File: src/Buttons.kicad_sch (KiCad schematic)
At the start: 23 parts

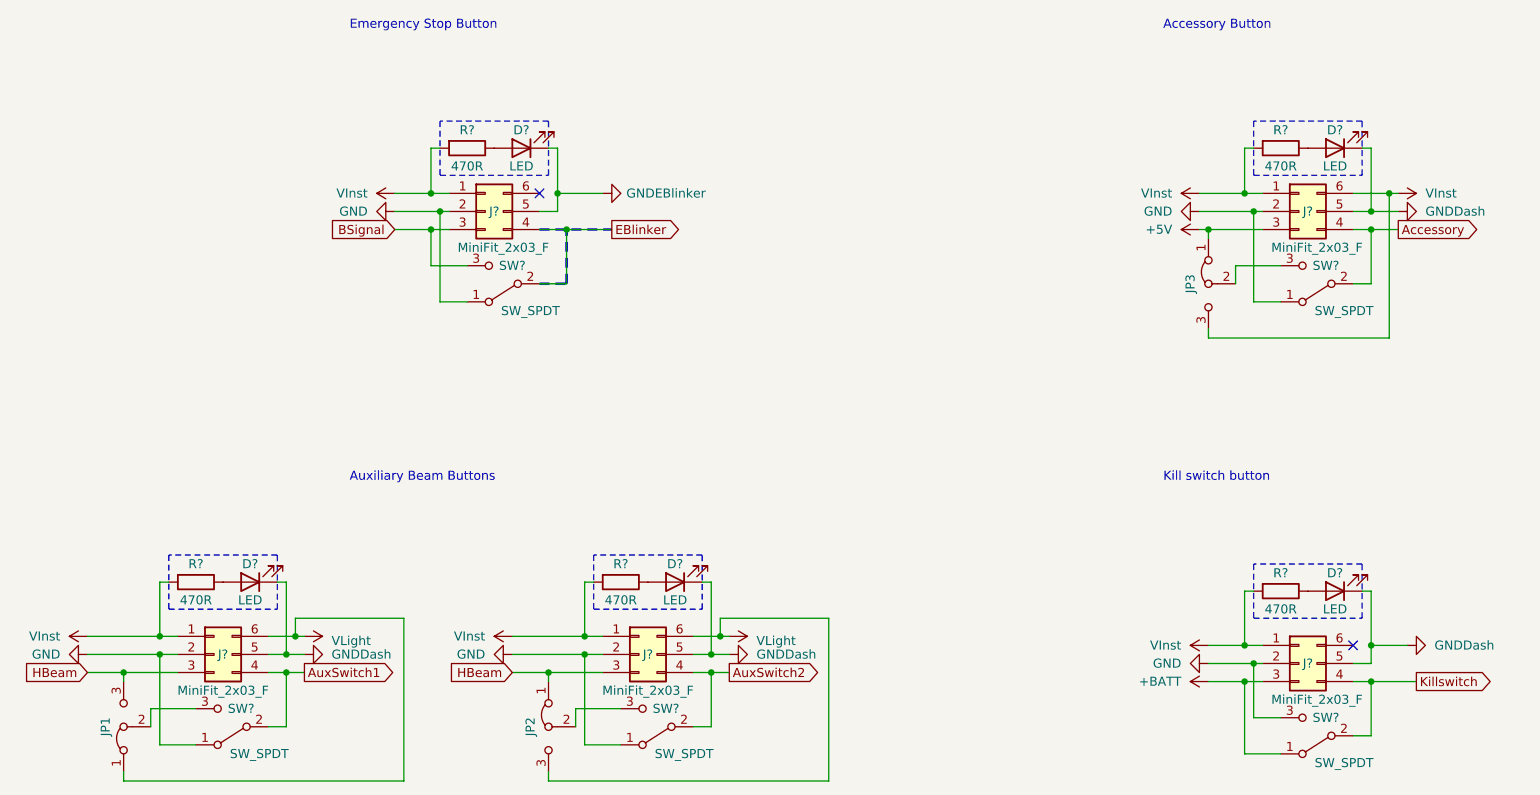
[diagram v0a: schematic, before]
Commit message: update Schematics
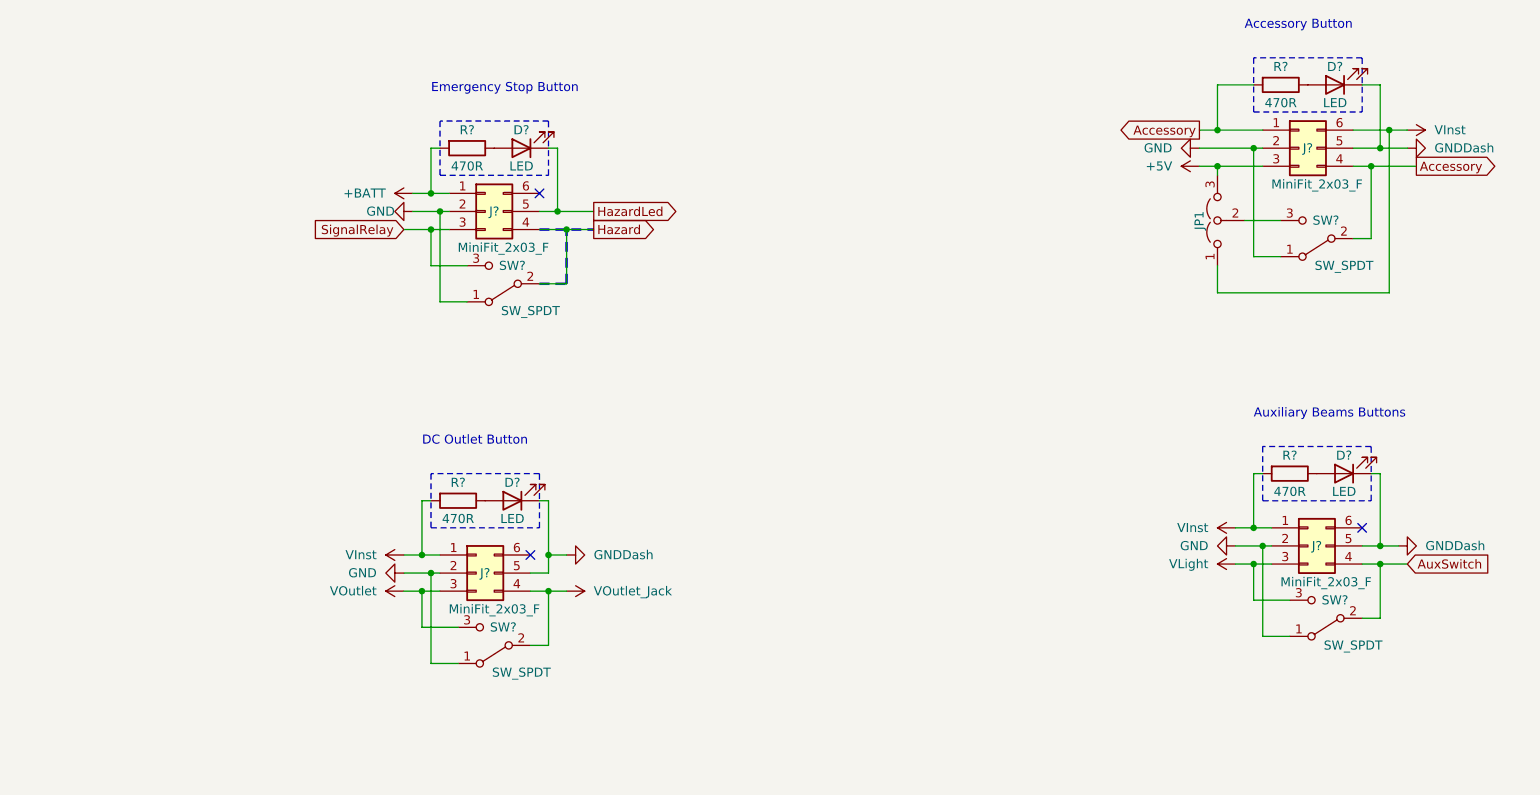
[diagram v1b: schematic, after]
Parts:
- removed D? (x2): LED, LED_THT:LED_D5.0mm, symbol Device:LED
- removed J? (x4): MiniFit_2x03_F, Connector_Molex:Molex_Mini-Fit_Jr_5566-06A_2x03_P4.20mm_Vertical, symbol Connector_Generic:Conn_02x03_Counter_Clockwise
- removed JP1, JP2, JP3: Jumper_3_Bridged12, symbol Jumper:Jumper_3_Bridged12
- removed R? (x2): 470R, Resistor_THT:R_Axial_DIN0204_L3.6mm_D1.6mm_P5.08mm_Horizontal, symbol Device:R
- removed SW? (x2): SW_SPDT, symbol Switch:SW_SPDT
- added D?: LED, LED_THT:LED_D5.0mm, symbol Device:LED
- added J? (x3): MiniFit_2x03_F, Connector_Molex:Molex_Mini-Fit_Jr_5566-06A_2x03_P4.20mm_Vertical, symbol Connector_Generic:Conn_02x03_Counter_Clockwise
- added JP1: Jumper_3_Open, symbol Jumper:Jumper_3_Open
- added R?: 470R, Resistor_THT:R_Axial_DIN0204_L3.6mm_D1.6mm_P5.08mm_Horizontal, symbol Device:R
- added SW?: SW_SPDT, symbol Switch:SW_SPDT
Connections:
- net +5V: now also J?.3 (Pin_3), JP1.3 (B)
- net +BATT: now also J?.1 (Pin_1), R?.2
- net Accessory: now also R?.2, J?.1 (Pin_1), J?.4 (Pin_4)
- net GND: now also J?.2 (Pin_2), J?.2 (Pin_2), J?.2 (Pin_2), SW?.1 (A)
- net GNDDash: now also D?.1 (K), J?.5 (Pin_5), J?.5 (Pin_5), J?.5 (Pin_5)
- net VInst: now also J?.1 (Pin_1), J?.1 (Pin_1), J?.6 (Pin_6), JP1.1 (A), R?.2; no longer J?.1 (Pin_1), R?.2, R?.2
- net VLight: now also SW?.3 (C), J?.3 (Pin_3)
- net at SW?.3 (C): now also JP1.2 (C)
- net AuxSwitch1 renamed AuxSwitch
- net AuxSwitch: now also J?.4 (Pin_4)
- net BSignal renamed SignalRelay
- net EBlinker renamed Hazard
- net GNDEBlinker renamed HazardLed
- new net: D?.2 (A), R?.1
- new net VOutlet: J?.3 (Pin_3), SW?.3 (C)
- new net VOutlet_Jack: J?.4 (Pin_4), SW?.2 (B)
- no-connect marks 2 -> 3
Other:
- note added: "Auxiliary Beams Buttons"
- note added: "DC Outlet Button"
- note removed: "Auxiliary Beam Buttons"
- note removed: "Kill switch button"
- moved on the sheet: D?, R?, SW?
